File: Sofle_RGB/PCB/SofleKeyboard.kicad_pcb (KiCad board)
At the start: 2 copper layers, 143.4 x 111.8 mm, 97 parts, among them J1 LED, J2 4PIN, J3 OLED, J4 key leds, J5 backlight sel, J6 indicator bypass, P1 i2c_pin, P2 i2c_pin, SW1 SW_PUSH-MX_W_LED, SW10 SW_PUSH-MX_W_LED, SW11 SW_PUSH-MX_W_LED, SW12 SW_PUSH-MX_W_LED, SW13 SW_PUSH-MX_W_LED, SW14 SW_PUSH-MX_W_LED, SW15 SW_PUSH-MX_W_LED, SW16 SW_PUSH-MX_W_LED, SW17 SW_PUSH-MX_W_LED, SW18 SW_PUSH-MX_W_LED, SW19 SW_PUSH-MX_W_LED, SW2 SW_PUSH-MX_W_LED, SW20 SW_PUSH-MX_W_LED, SW21 SW_PUSH-MX_W_LED, SW22 SW_PUSH-MX_W_LED, SW23 SW_PUSH-MX_W_LED, SW24 SW_PUSH-MX_W_LED, SW25 Rotary_Encoder_Switch, SW26 SW_PUSH-MX_W_LED, SW27 SW_PUSH-MX_W_LED, SW28 SW_PUSH-MX_W_LED, SW29 SW_PUSH-MX_W_LED, SW3 SW_PUSH-MX_W_LED, SW30 SW_PUSH-MX_W_LED, SW4 SW_PUSH-MX_W_LED, SW5 SW_PUSH-MX_W_LED, SW6 SW_PUSH-MX_W_LED, SW7 SW_PUSH-MX_W_LED, SW8 SW_PUSH-MX_W_LED, SW9 SW_PUSH-MX_W_LED, U1 ProMicro

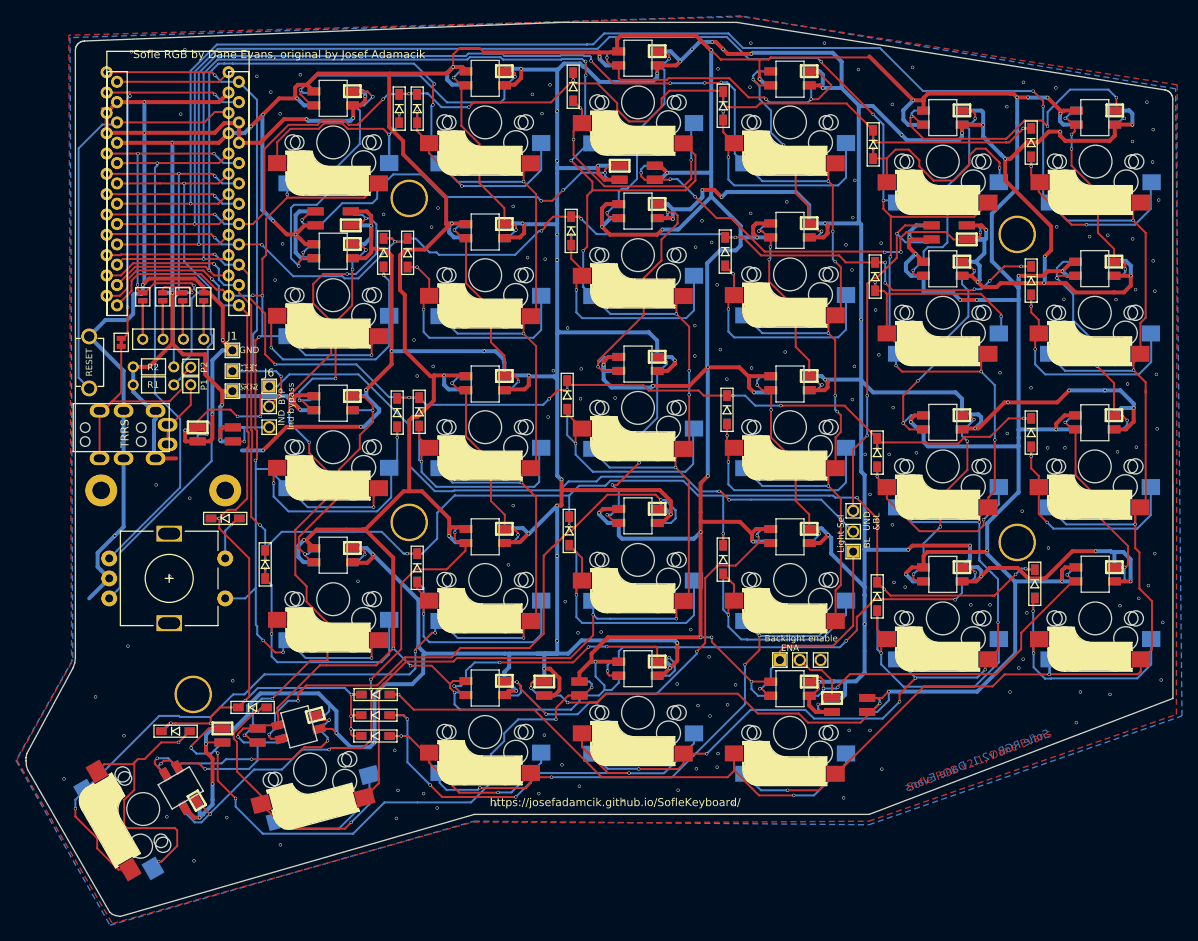
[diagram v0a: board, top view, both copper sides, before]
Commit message: Current progress in RP2040 design
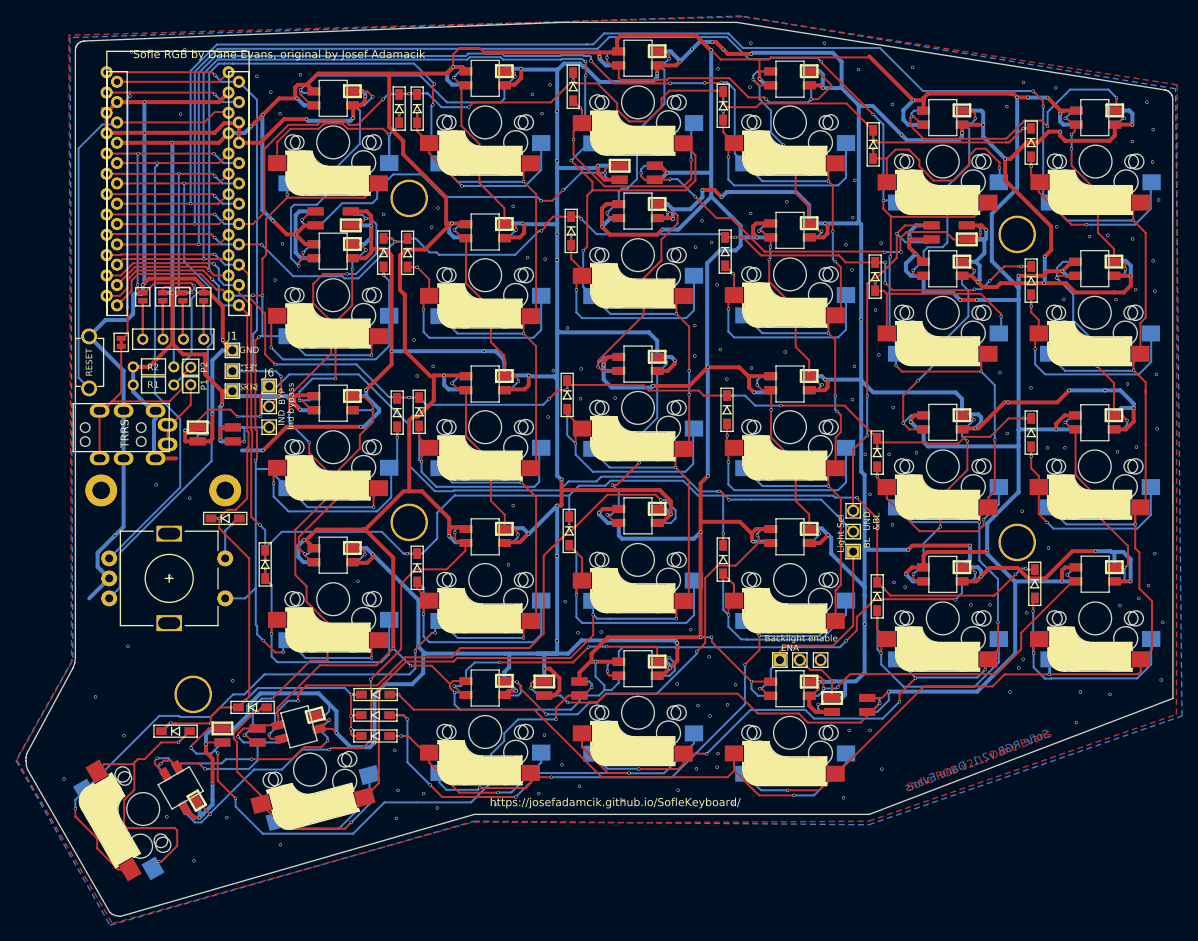
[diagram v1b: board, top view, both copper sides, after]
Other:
- net class Default removed
- net class GND removed
- net class VCC removed
